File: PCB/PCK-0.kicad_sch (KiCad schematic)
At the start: 88 parts, among them J1 USB_C_Receptacle_USB2.0_16P, J2 BAT+, J3 BAT-, SW1 1,1, SW10 3,2, SW11 4,2, SW12 5,2, SW13 6,2, SW14 7,2, SW15 EN, SW16 1,3, SW17 2,3, SW18 3,3, SW19 4,3, SW2 2,1, SW20 5,3, SW21 6,3, SW22 7,3, SW23 1,4, SW24 2,4, SW25 3,4, SW26 4,4, SW27 5,4, SW28 6,4, SW29 7,4, SW3 3,1, SW30 BOOT, SW31 RotaryEncoder_Switch_MP, SW4 4,1, SW5 5,1, SW6 6,1, SW7 7,1, SW8 1,2, SW9 2,2, U1 NCP1117-3.3_SOT223, U2 NCP1117-3.3_SOT223, U3 USBLC6-2SC6, U4 ESP32-C6-MINI-1, U5 TVS1400DRV

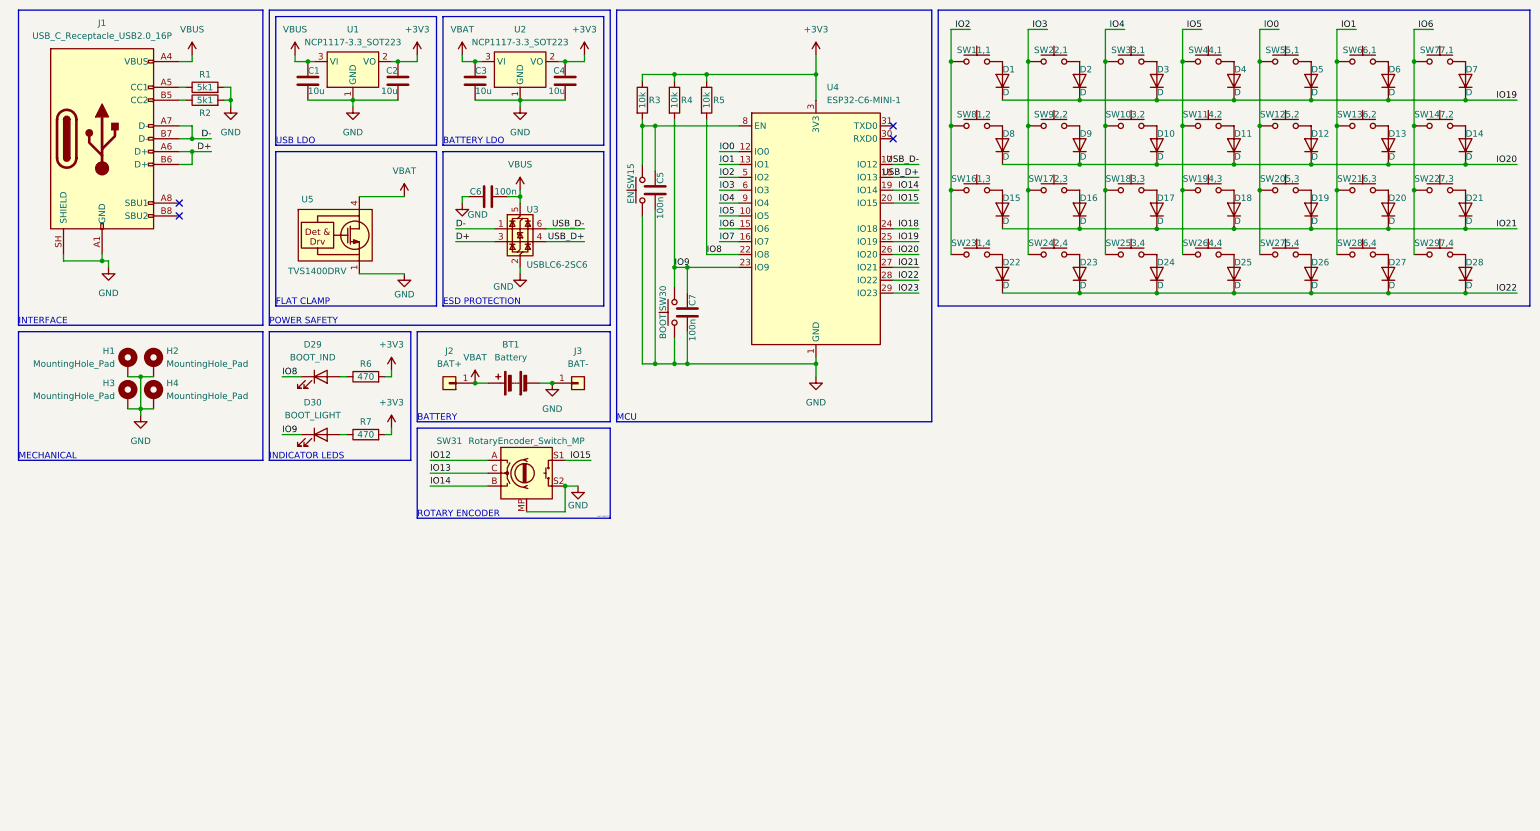
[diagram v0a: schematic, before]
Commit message: one must imagine sisyphus happy
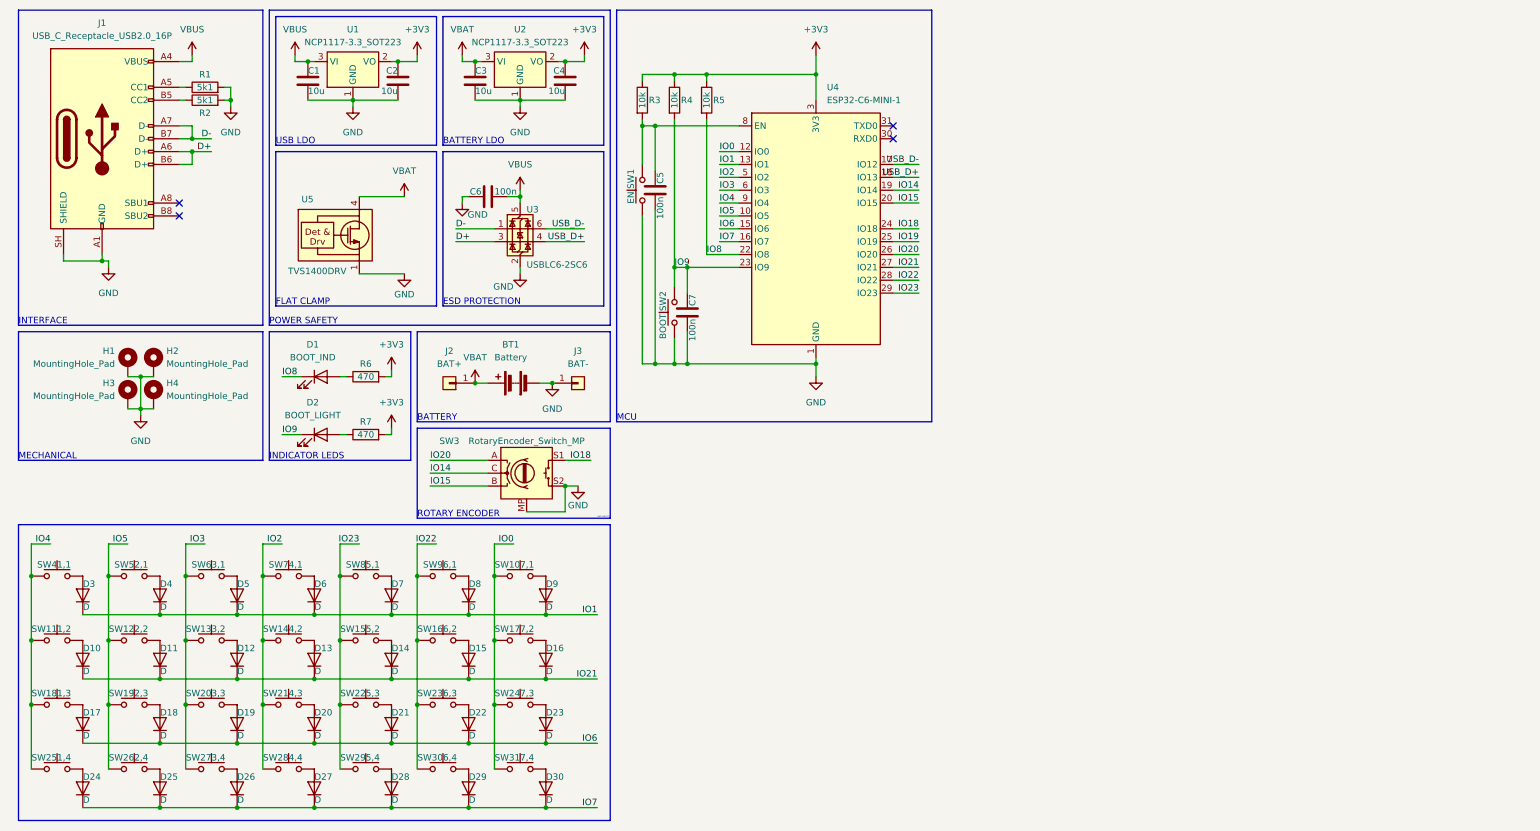
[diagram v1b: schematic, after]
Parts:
- renumbered D29 to D1, D8 to D10, D9 to D11, D10 to D12, D11 to D13, D12 to D14, D13 to D15, D14 to D16, D15 to D17, D16 to D18, D17 to D19, D30 to D2, D18 to D20, D19 to D21, D20 to D22, D21 to D23, D22 to D24, D23 to D25, D24 to D26, D25 to D27, D26 to D28, D27 to D29, D1 to D3, D28 to D30, D2 to D4, D3 to D5, D4 to D6, D5 to D7, D6 to D8, D7 to D9, SW15 to SW1, SW7 to SW10, SW8 to SW11, SW9 to SW12, SW10 to SW13, SW11 to SW14, SW12 to SW15, SW13 to SW16, SW14 to SW17, SW16 to SW18, SW17 to SW19, SW30 to SW2, SW18 to SW20, SW19 to SW21, SW20 to SW22, SW21 to SW23, SW22 to SW24, SW23 to SW25, SW24 to SW26, SW25 to SW27, SW26 to SW28, SW27 to SW29, SW31 to SW3, SW28 to SW30, SW29 to SW31, SW1 to SW4, SW2 to SW5, SW3 to SW6, SW4 to SW7, SW5 to SW8, SW6 to SW9
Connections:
- net IO12 is gone; now on net IO20: SW3.A
- net IO13 is gone; now on net IO14: SW3.C
- net IO0: now also SW10.1, SW17.1, SW24.1, SW31.1; no longer SW15.1, SW22.1, SW29.1, SW8.1
- net IO1: now also D3.1 (K), D4.1 (K), D5.1 (K), D6.1 (K), D7.1 (K), D8.1 (K), D9.1 (K); no longer SW16.1, SW23.1, SW30.1, SW9.1
- net IO14: no longer SW3.B
- net IO15: now also SW3.B; no longer SW3.S1
- net IO18: now also SW3.S1
- net IO19: no longer D3.1 (K), D4.1 (K), D5.1 (K), D6.1 (K), D7.1 (K), D8.1 (K), D9.1 (K)
- net IO2: now also SW14.1, SW21.1, SW28.1, SW7.1; no longer SW11.1, SW18.1, SW25.1, SW4.1
- net IO20: no longer D10.1 (K), D11.1 (K), D12.1 (K), D13.1 (K), D14.1 (K), D15.1 (K), D16.1 (K)
- net IO21: now also D10.1 (K), D11.1 (K), D12.1 (K), D13.1 (K), D14.1 (K), D15.1 (K), D16.1 (K); no longer D17.1 (K), D18.1 (K), D19.1 (K), D20.1 (K), D21.1 (K), D22.1 (K), D23.1 (K)
- net IO22: now also SW16.1, SW23.1, SW30.1, SW9.1; no longer D24.1 (K), D25.1 (K), D26.1 (K), D27.1 (K), D28.1 (K), D29.1 (K), D30.1 (K)
- net IO23: now also SW15.1, SW22.1, SW29.1, SW8.1
- net IO3: now also SW13.1, SW20.1, SW27.1, SW6.1; no longer SW12.1, SW19.1, SW26.1, SW5.1
- net IO4: now also SW11.1, SW18.1, SW25.1, SW4.1; no longer SW13.1, SW20.1, SW27.1, SW6.1
- net IO5: now also SW12.1, SW19.1, SW26.1, SW5.1; no longer SW14.1, SW21.1, SW28.1, SW7.1
- net IO6: now also D17.1 (K), D18.1 (K), D19.1 (K), D20.1 (K), D21.1 (K), D22.1 (K), D23.1 (K); no longer SW10.1, SW17.1, SW24.1, SW31.1
- net IO7: now also D24.1 (K), D25.1 (K), D26.1 (K), D27.1 (K), D28.1 (K), D29.1 (K), D30.1 (K)
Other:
- moved on the sheet: D10, D11, D12, D13, D14, D15, D16, D17, D18, D19, D20, D21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
